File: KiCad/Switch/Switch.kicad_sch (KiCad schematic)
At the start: 48 parts, among them Q1 BD139, Q2 IXTH90P10P, Q4 BD139, Q5A1 BSC340N08NS3G, Q6 BD139, U1 AD8033

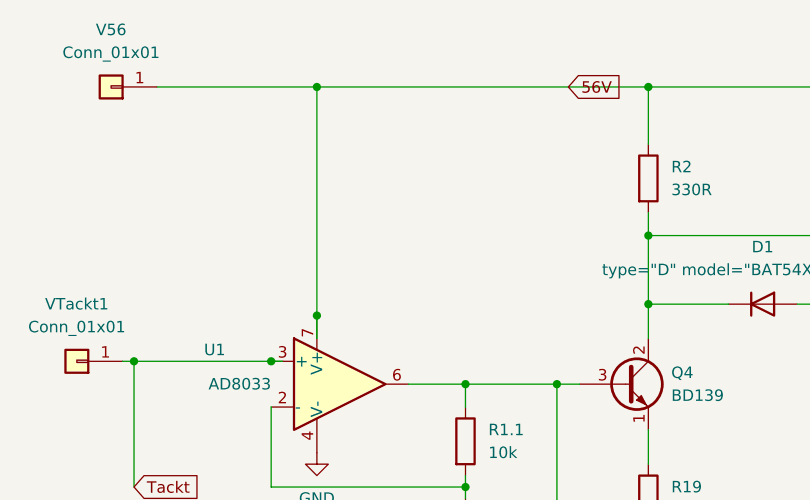
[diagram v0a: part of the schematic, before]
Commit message: Simulation und PCB update
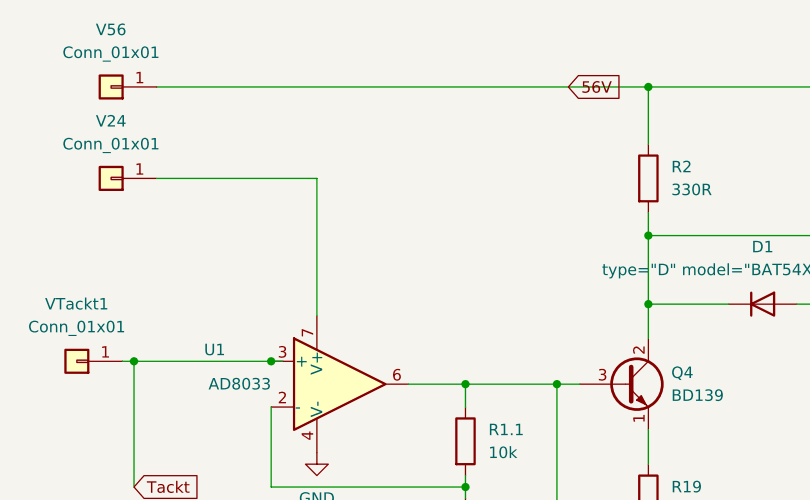
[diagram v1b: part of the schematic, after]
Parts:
- added V24: Conn_01x01, Connector:Banana_Jack_1Pin, symbol Connector_Generic:Conn_01x01
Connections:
- net 56V: no longer U1.7 (V+)
- new net: U1.7 (V+), V24.1 (Pin_1)
